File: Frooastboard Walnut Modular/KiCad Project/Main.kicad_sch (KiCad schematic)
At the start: 215 parts, among them J10 F Row CS, J11 F Row SW, J15 F Row, J16 F Row USB, J17 Numpad, J8 Numpad CS, J9 Numpad SW, M2 Frooastboard_MM2040

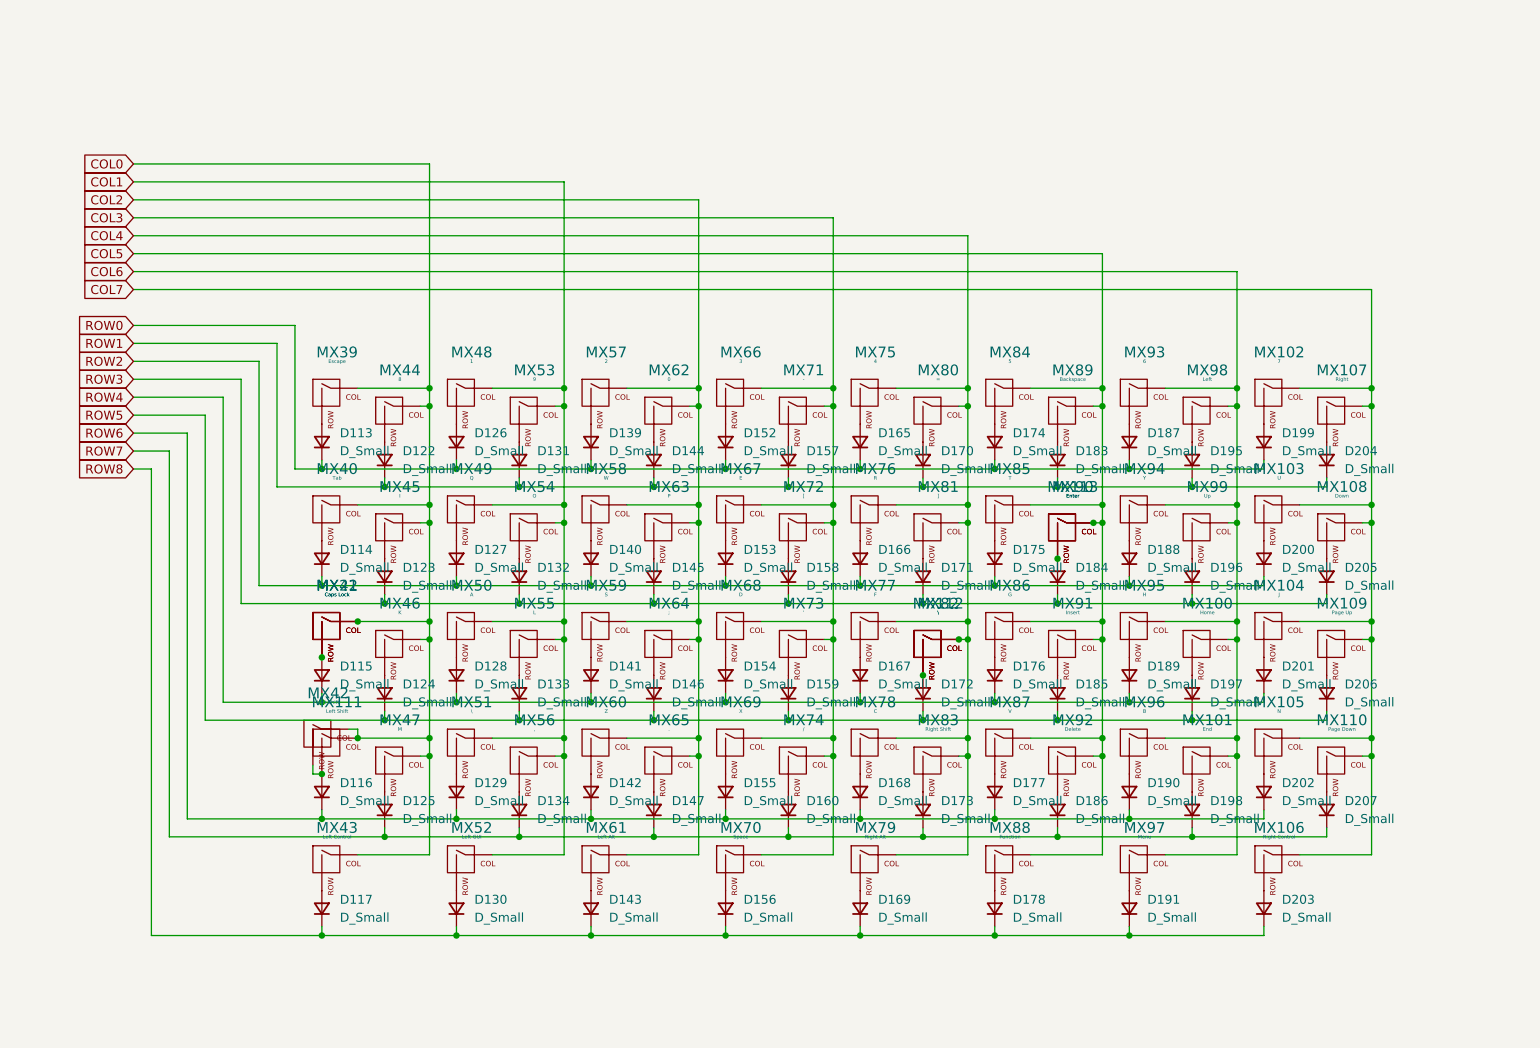
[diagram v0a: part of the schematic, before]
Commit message: all keys placed
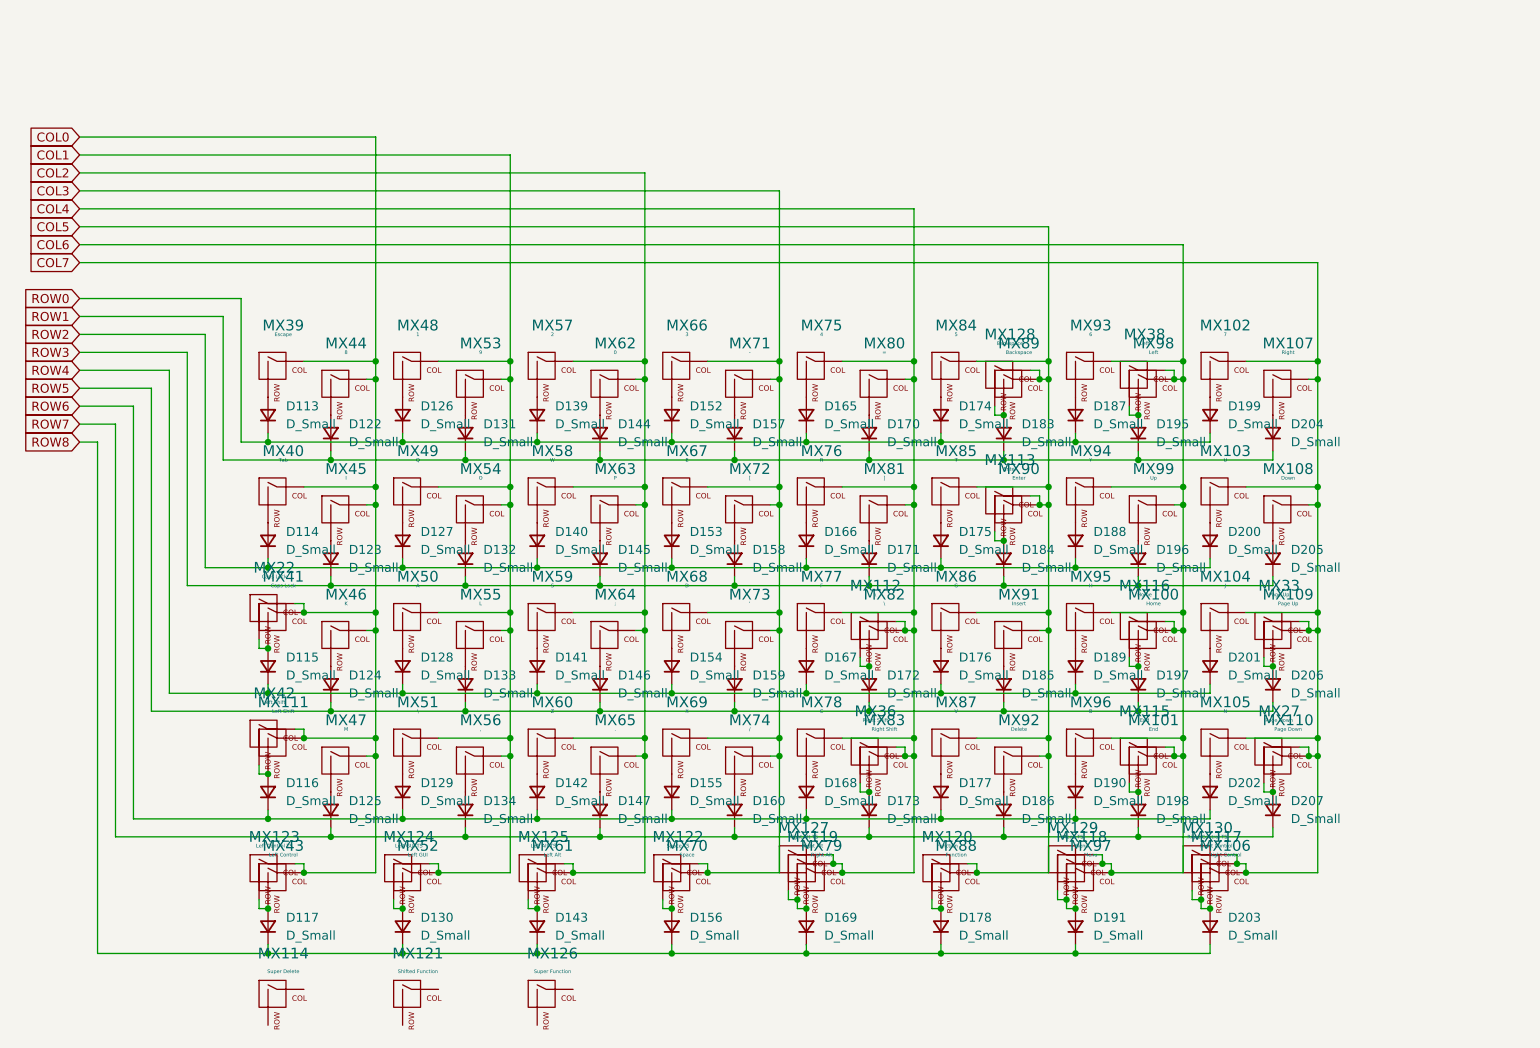
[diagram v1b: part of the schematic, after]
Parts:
- added MX114: Super Delete, MX_Only:MXOnly-1U-NoLED, symbol MX_Alps_Hybrid:MX-NoLED
- added MX115: End, MX_Only:MXOnly-1U-NoLED, symbol MX_Alps_Hybrid:MX-NoLED
- added MX116: Home, MX_Only:MXOnly-1U-NoLED, symbol MX_Alps_Hybrid:MX-NoLED
- added MX117: Right Control, MX_Only:MXOnly-1U-NoLED, symbol MX_Alps_Hybrid:MX-NoLED
- added MX118: Menu, MX_Only:MXOnly-1U-NoLED, symbol MX_Alps_Hybrid:MX-NoLED
- added MX119: Right Alt, MX_Only:MXOnly-1U-NoLED, symbol MX_Alps_Hybrid:MX-NoLED
- added MX120: Function, MX_Only:MXOnly-1U-NoLED, symbol MX_Alps_Hybrid:MX-NoLED
- added MX121: Shifted Function, MX_Only:MXOnly-1U-NoLED, symbol MX_Alps_Hybrid:MX-NoLED
- added MX122: Space TS, MX_Only:MXOnly-7U-ReversedStabilizers-NoLED, symbol MX_Alps_Hybrid:MX-NoLED
- added MX123: Left Control TS, MX_Only:MXOnly-1.5U-NoLED, symbol MX_Alps_Hybrid:MX-NoLED
- added MX124: Left GUI TS, MX_Only:MXOnly-1U-NoLED, symbol MX_Alps_Hybrid:MX-NoLED
- added MX125: Left Alt TS, MX_Only:MXOnly-1.5U-NoLED, symbol MX_Alps_Hybrid:MX-NoLED
- added MX126: Super Function, MX_Only:MXOnly-1U-NoLED, symbol MX_Alps_Hybrid:MX-NoLED
- added MX127: Right Alt TS, MX_Only:MXOnly-1.5U-NoLED, symbol MX_Alps_Hybrid:MX-NoLED
- added MX128: Backspace, MX_Only:MXOnly-1U-NoLED, symbol MX_Alps_Hybrid:MX-NoLED
- added MX129: Menu TS, MX_Only:MXOnly-1U-NoLED, symbol MX_Alps_Hybrid:MX-NoLED
- added MX130: Right Control TS, MX_Only:MXOnly-1.5U-NoLED, symbol MX_Alps_Hybrid:MX-NoLED
- added MX27: Page Down, MX_Only:MXOnly-1U-NoLED, symbol MX_Alps_Hybrid:MX-NoLED
- added MX33: Page Up, MX_Only:MXOnly-1U-NoLED, symbol MX_Alps_Hybrid:MX-NoLED
- added MX36: Right Shift, MX_Only:MXOnly-1.75U-NoLED, symbol MX_Alps_Hybrid:MX-NoLED
- added MX38: Left, MX_Only:MXOnly-1U-NoLED, symbol MX_Alps_Hybrid:MX-NoLED
- MX90: footprint MX_Only:MXOnly-ISO-ROTATED-NoLED-NoStabilizers -> MX_Only:MXOnly-ISO-ROTATED-NoLED
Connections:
- net COL0: now also MX123.1 (COL)
- net COL1: now also MX124.1 (COL)
- net COL2: now also MX125.1 (COL)
- net COL3: now also MX122.1 (COL)
- net COL4: now also MX119.1 (COL), MX127.1 (COL), MX36.1 (COL)
- net COL5: now also MX120.1 (COL), MX128.1 (COL)
- net COL6: now also MX115.1 (COL), MX116.1 (COL), MX118.1 (COL), MX129.1 (COL), MX38.1 (COL)
- net COL7: now also MX117.1 (COL), MX130.1 (COL), MX27.1 (COL), MX33.1 (COL)
- net at D183.2 (A), MX89.2 (ROW): now also MX128.2 (ROW)
- net at D191.2 (A), MX97.2 (ROW): now also MX118.2 (ROW), MX129.2 (ROW)
- net at D169.2 (A), MX79.2 (ROW): now also MX119.2 (ROW), MX127.2 (ROW)
- net at D117.2 (A), MX43.2 (ROW): now also MX123.2 (ROW)
- net at D203.2 (A), MX106.2 (ROW): now also MX117.2 (ROW), MX130.2 (ROW)
- net at D195.2 (A), MX98.2 (ROW): now also MX38.2 (ROW)
- net at D173.2 (A), MX83.2 (ROW): now also MX36.2 (ROW)
- net at D198.2 (A), MX101.2 (ROW): now also MX115.2 (ROW)
- net at D206.2 (A), MX109.2 (ROW): now also MX33.2 (ROW)
- net at D143.2 (A), MX61.2 (ROW): now also MX125.2 (ROW)
- net at D197.2 (A), MX100.2 (ROW): now also MX116.2 (ROW)
- net at D178.2 (A), MX88.2 (ROW): now also MX120.2 (ROW)
- net at D156.2 (A), MX70.2 (ROW): now also MX122.2 (ROW)
- net at D130.2 (A), MX52.2 (ROW): now also MX124.2 (ROW)
- net at D207.2 (A), MX110.2 (ROW): now also MX27.2 (ROW)
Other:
- moved on the sheet: D113, D114, D115, D116, D117, D122, D123, D124, D125, D126, D127, D128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
